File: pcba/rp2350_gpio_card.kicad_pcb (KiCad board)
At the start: 2 copper layers, 26 x 30 mm, 41 parts, among them J1 Conn_01x10_Pin, J2 Conn_01x10_Pin, P1 USB_C_Plug_USB2.0, U1 RP2350_60QFN, U2 W25Q128JVS, U4 AP2127K-3.3, Y1 ABM8-272-T3

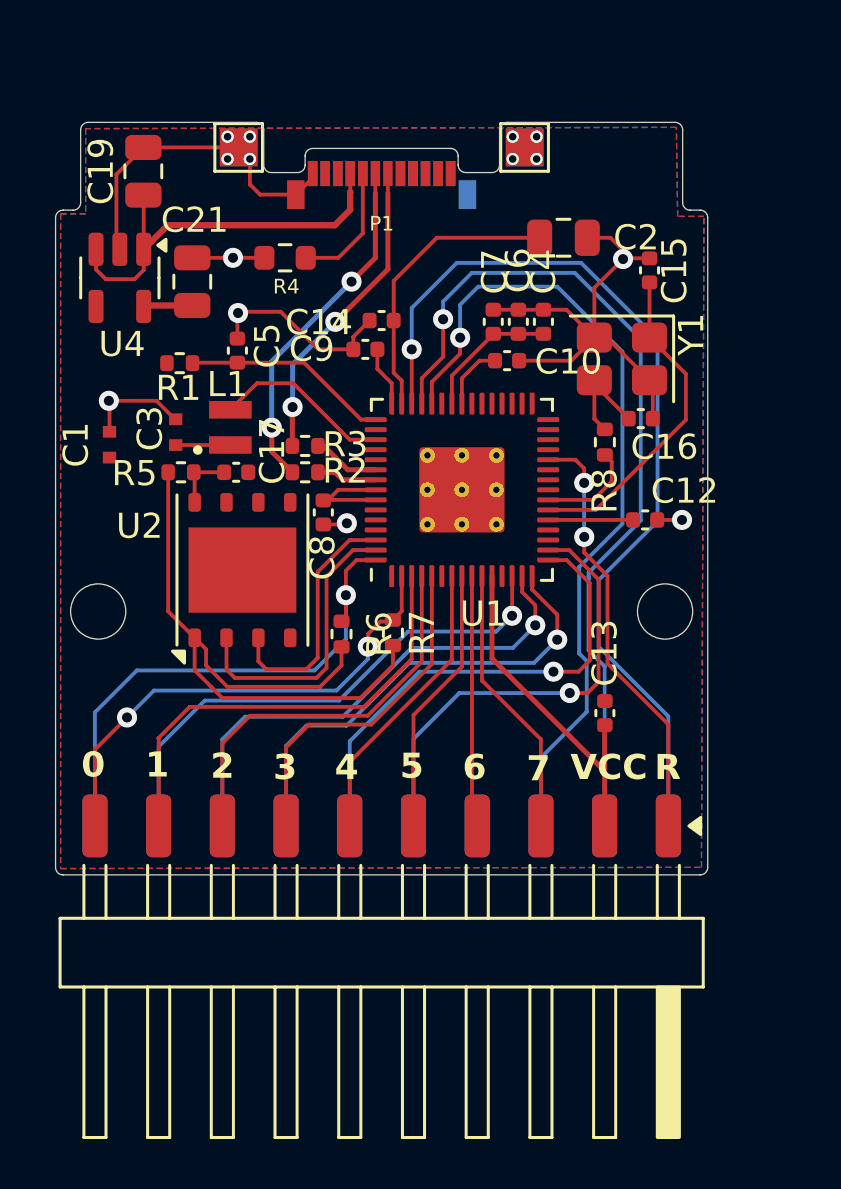
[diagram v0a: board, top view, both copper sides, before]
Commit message: add copyright claim
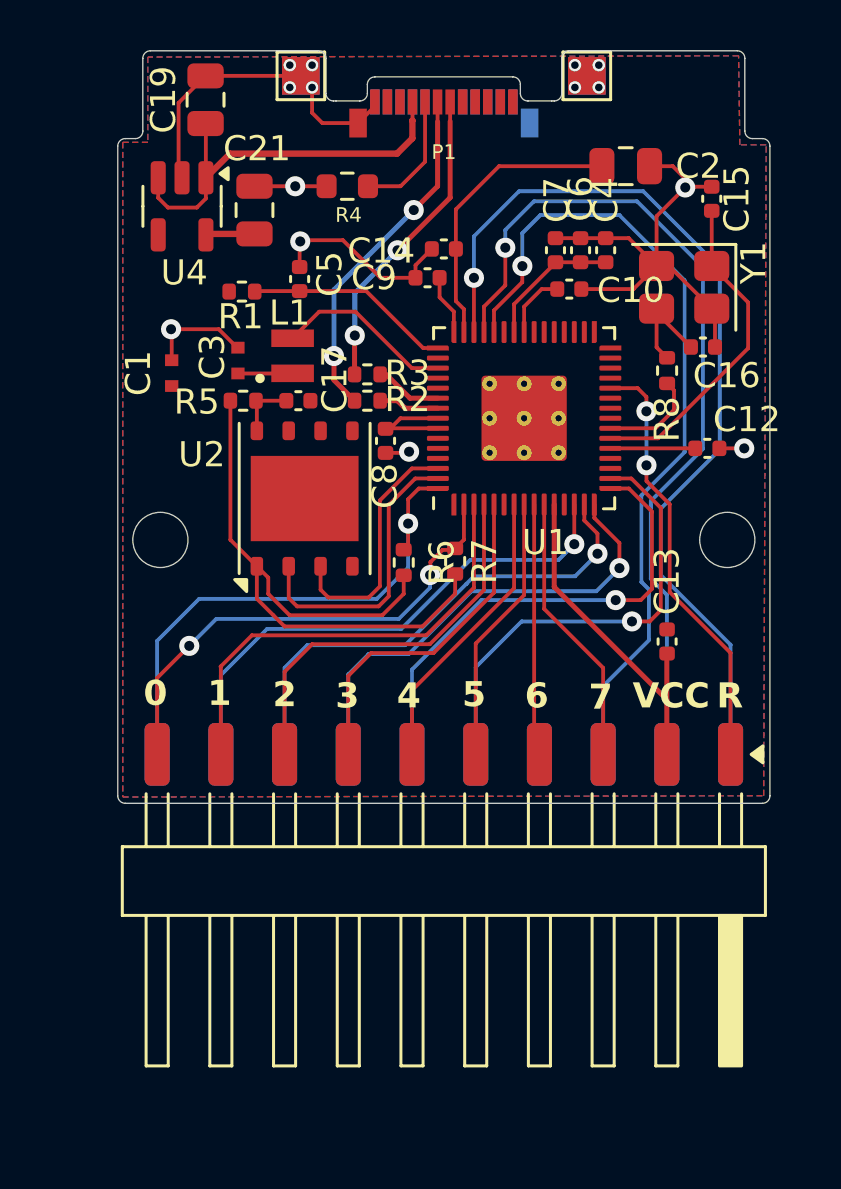
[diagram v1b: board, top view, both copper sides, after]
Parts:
- moved C1 3.78 mm to (92.7, 65.0)
- moved C13 3.78 mm to (112.5, 75.7)
- moved C15 3.78 mm to (114.2, 58.0)
- moved C3 3.78 mm to (95.3, 64.5)
- moved R4 3.78 mm to (99.7, 57.5)
- moved R6 3.78 mm to (102.0, 72.5)
- moved R8 3.78 mm to (112.5, 64.9)
- moved Y1 3.78 mm to (113.1, 61.6)
- moved C10 3.78 mm to (108.6, 61.6)
- moved C12 3.78 mm to (114.1, 68.0)
- moved C14 3.78 mm to (103.6, 60.0)
- moved C16 3.78 mm to (113.9, 64.0)
- moved C17 3.78 mm to (97.8, 66.1)
- moved C19 3.78 mm to (94.1, 54.1)
- moved C2 3.78 mm to (110.8, 56.7)
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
